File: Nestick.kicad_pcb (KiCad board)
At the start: 2 copper layers, 20 parts, among them J1 CONN_EXT, J2 CONN_DIRS, J3 CONN_DGND, J4 CONN_BTNS, J5 CONN_BGND, Q1 2N3904, U1 74LS165, U2 74LS165

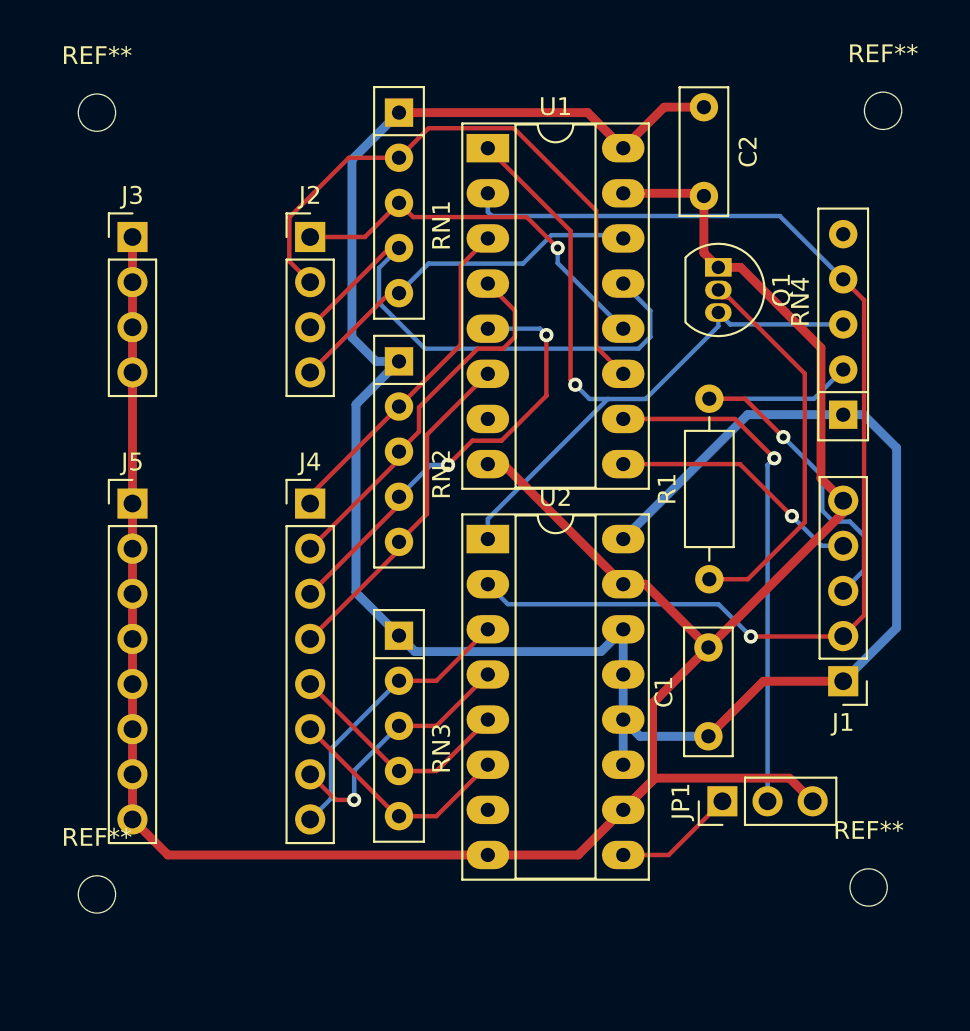
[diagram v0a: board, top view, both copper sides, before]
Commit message: Dress up for release
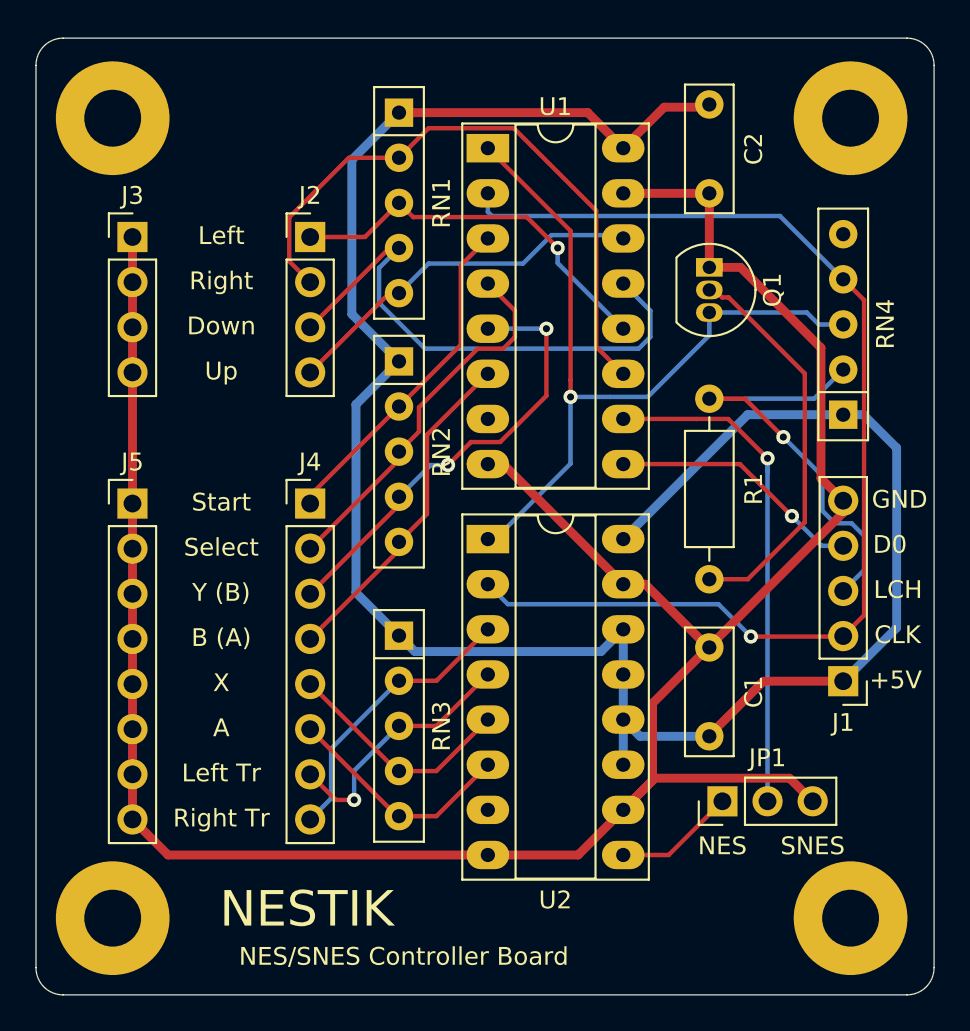
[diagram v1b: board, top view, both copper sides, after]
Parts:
- removed REF** (x4): MountingHole_2.1mm, MountingHole:MountingHole_2.1mm
- added H1: HOLE, MountingHole:MountingHole_3.2mm_M3_Pad, F.Cu at (103.9, 148.3)
- added H2: HOLE, MountingHole:MountingHole_3.2mm_M3_Pad, F.Cu at (145.4, 148.3)
- added H3: HOLE, MountingHole:MountingHole_3.2mm_M3_Pad, F.Cu at (145.4, 103.3)
- added H4: HOLE, MountingHole:MountingHole_3.2mm_M3_Pad, F.Cu at (103.9, 103.3)
- moved Q1 0.51 mm to (137.5, 111.7)
- moved C2 0.34 mm to (137.5, 102.5)
- moved C1 0.05 mm to (137.5, 138.1)
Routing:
- net VCC: track 122.0 -> 121.2 mm
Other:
- board outline added: 50.5 x 53.8 mm
- board text added: "+5V"
- board text added: "B (A)"
- board text added: "CLK"
- board text added: "D0"
- board text added: "GND"
- board text added: "LCH"
- board text added: "NES"
- board text added: "NES/SNES Controller Board"
- board text added: "NESTIK"
- board text added: "SNES"
- board text added: "Y (B)"
- board text removed: "B"
- board text removed: "Y"
